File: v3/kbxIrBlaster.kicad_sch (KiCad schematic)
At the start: 46 parts, among them J1 CH1, J2 CH2, J3 CH3, J4 CH4, J5 Conn_01x06, J6 Conn_01x15, J7 Conn_01x15, J8 Barrel_Jack_Switch, J9 USB_B_Micro, Q1 2N7002, Q2 2N7002, Q3 2N7002, Q4 2N7002, SW1 RESET, SW2 BOOT, U1 TSOP382xx, U2 TSOP382xx, U3 ESP32-WROOM-32D, U4 AP2112K-3.3

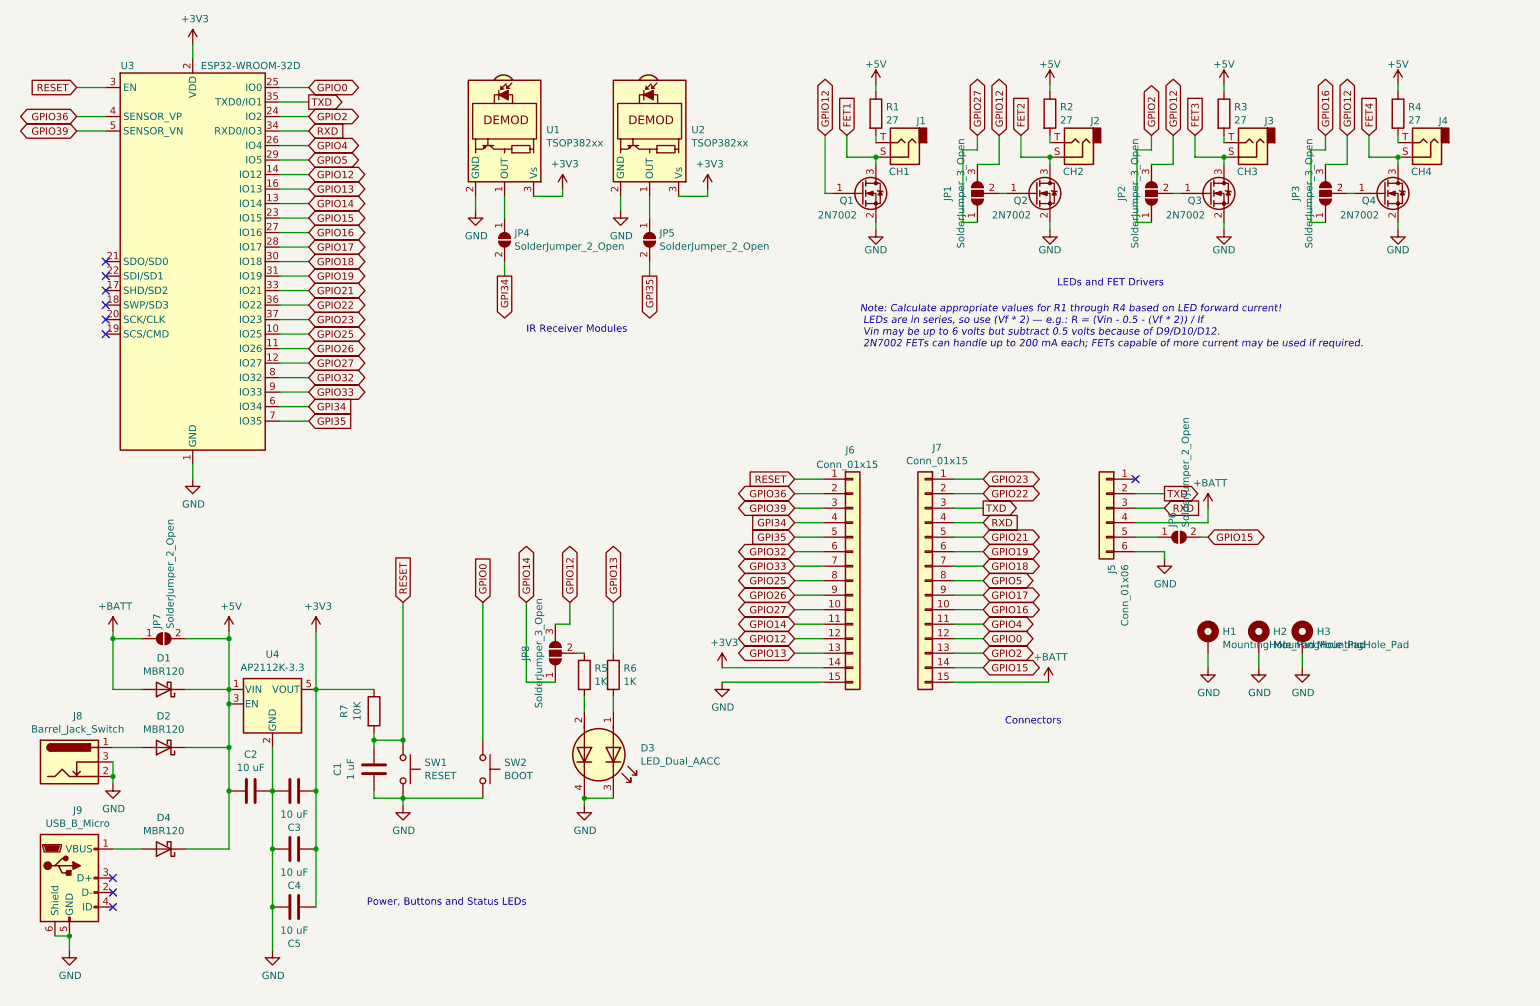
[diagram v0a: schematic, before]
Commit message: Update with v3
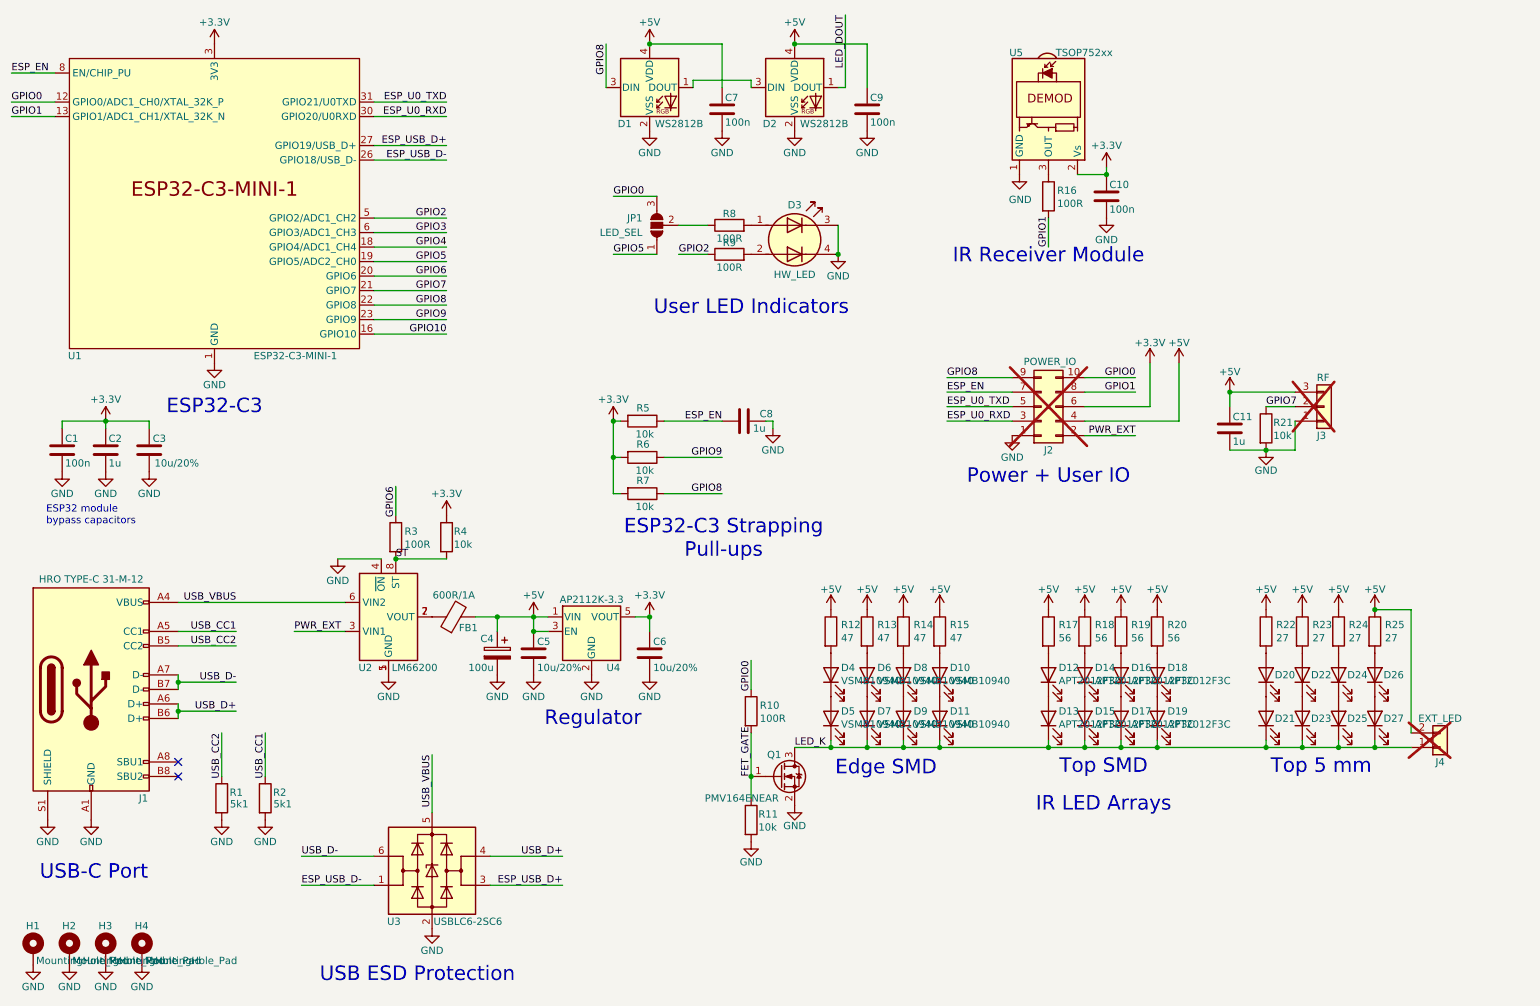
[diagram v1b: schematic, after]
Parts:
- removed C4: 10 uF, Capacitor_SMD:C_0805_2012Metric_Pad1.18x1.45mm_HandSolder, symbol Device:C
- removed D1, D2, D4: MBR120, Diode_SMD:D_SOD-123F, symbol Device:D_Schottky
- removed D3: LED_Dual_AACC, LED_SMD:LED_Cree-PLCC4_3.2x2.8mm_CCW, symbol Device:LED_Dual_AACC
- removed J1: CH1, Connector_Audio:Jack_3.5mm_CUI_SJ1-3533NG_Horizontal, symbol Connector:AudioJack2
- removed J2: CH2, Connector_Audio:Jack_3.5mm_CUI_SJ1-3533NG_Horizontal, symbol Connector:AudioJack2
- removed J3: CH3, Connector_Audio:Jack_3.5mm_CUI_SJ1-3533NG_Horizontal, symbol Connector:AudioJack2
- removed J4: CH4, Connector_Audio:Jack_3.5mm_CUI_SJ1-3533NG_Horizontal, symbol Connector:AudioJack2
- removed J5: Conn_01x06, Connector_PinHeader_2.54mm:PinHeader_1x06_P2.54mm_Vertical, symbol Connector_Generic:Conn_01x06
- removed J6, J7: Conn_01x15, Connector_PinHeader_2.54mm:PinHeader_1x15_P2.54mm_Vertical, symbol Connector_Generic:Conn_01x15
- removed J8: Barrel_Jack_Switch, Connector_BarrelJack:BarrelJack_Horizontal, symbol Connector:Barrel_Jack_Switch
- removed J9: USB_B_Micro, Connector_USB:USB_Micro-B_Molex-105017-0001, symbol Connector:USB_B_Micro
- removed JP2, JP3, JP8: SolderJumper_3_Open, Jumper:SolderJumper-3_P1.3mm_Open_RoundedPad1.0x1.5mm, symbol Jumper:SolderJumper_3_Open
- removed JP4, JP5, JP6, JP7: SolderJumper_2_Open, Jumper:SolderJumper-2_P1.3mm_Open_RoundedPad1.0x1.5mm, symbol Jumper:SolderJumper_2_Open
- removed Q2, Q3, Q4: 2N7002, Package_TO_SOT_SMD:SOT-23, symbol Transistor_FET:2N7002
- removed SW1: RESET, Button_Switch_SMD:SW_Push_1P1T_NO_CK_KMR2, symbol Switch:SW_Push
- removed SW2: BOOT, Button_Switch_SMD:SW_Push_1P1T_NO_CK_KMR2, symbol Switch:SW_Push
- removed U1, U2: TSOP382xx, OptoDevice:Vishay_MINICAST-3Pin, symbol Interface_Optical:TSOP382xx
- removed U3: ESP32-WROOM-32D, RF_Module:ESP32-WROOM-32, symbol RF_Module:ESP32-WROOM-32D
- added C10, C7, C9: 100n, Capacitor_SMD:C_0402_1005Metric, symbol Device:C
- added C11, C8: 1u, Capacitor_SMD:C_0402_1005Metric, symbol Device:C
- added C4: 100u, Capacitor_SMD:CP_Elec_5x5.4, symbol Device:CP
- added C6: 10u/20%, Capacitor_SMD:C_0603_1608Metric, symbol Device:C
- added D1, D2: WS2812B, LED_SMD:LED_WS2812B-2020_PLCC4_2.0x2.0mm, symbol Pulse:WS2812B
- added D10, D11, D4, D5, D6, D7, D8, D9: VSMB10940, LED_SMD:LED_Kingbright_KPA-3010_3x2x1mm, symbol Device:LED
- added D12, D13, D14, D15, D16, D17, D18, D19: APT2012F3C, LED_SMD:LED_0805_2012Metric, symbol Device:LED
- added D20, D21, D22, D23, D24, D25, D26, D27: CH1, LED_THT:LED_D5.0mm, symbol Device:LED
- added D3: HW_LED, LED_SMD:LED_Cree-PLCC4_3.2x2.8mm_CCW, symbol Device:LED_Dual_AAKK
- added FB1: 600R/1A, Inductor_SMD:L_0603_1608Metric, symbol Device:FerriteBead
- added H4: MountingHole_Pad, MountingHole:MountingHole_2.5mm_Pad_Via, symbol Mechanical:MountingHole_Pad
- added J1: HRO TYPE-C 31-M-12, Connector_USB:USB_C_Receptacle_HRO_TYPE-C-31-M-12, symbol Connector:USB_C_Receptacle_USB2.0
- added J2: POWER_IO, Connector_PinSocket_2.54mm:PinSocket_2x05_P2.54mm_Vertical, symbol Connector_Generic:Conn_02x05_Odd_Even
- added J3: RF, Connector_PinSocket_2.54mm:PinSocket_1x03_P2.54mm_Vertical, symbol Connector_Generic:Conn_01x03
- added J4: EXT_LED, Connector_PinSocket_2.54mm:PinSocket_1x02_P2.54mm_Vertical, symbol Connector_Generic:Conn_01x02
- added R10, R16, R8, R9: 100R, Resistor_SMD:R_0402_1005Metric, symbol Device:R
- added R11, R21: 10k, Resistor_SMD:R_0402_1005Metric, symbol Device:R
- added R12, R13, R14, R15: 47, Resistor_SMD:R_0805_2012Metric, symbol Device:R
- added R17, R18, R19, R20: 56, Resistor_SMD:R_0805_2012Metric, symbol Device:R
- added R22, R23, R24, R25: 27, Resistor_SMD:R_0805_2012Metric, symbol Device:R
- added U1: ESP32-C3-MINI-1, PCM_Espressif:ESP32-C3-MINI-1, symbol PCM_Espressif:ESP32-C3-MINI-1
- added U2: LM66200, Package_TO_SOT_SMD:SOT-583-8, symbol kbxIrBlaster:LM66200
- added U3: USBLC6-2SC6, Package_TO_SOT_SMD:SOT-23-6, symbol Power_Protection:USBLC6-2SC6
- added U5: TSOP752xx, kbxIrBlaster:Vishay_TSOP752_Horizontal, symbol kbxIrBlaster:TSOP752xx
- C1: value 1 uF -> 100n; footprint Capacitor_SMD:C_0805_2012Metric_Pad1.18x1.45mm_HandSolder -> Capacitor_SMD:C_0402_1005Metric; DesignRef (none) -> Bypass; MPN1 C0805C105K4RACTU -> CC0402KRX5R6BB104; MPN2 - -> (none); Manufacturer (none) -> Yageo
- C2: value 10 uF -> 1u; footprint Capacitor_SMD:C_0805_2012Metric_Pad1.18x1.45mm_HandSolder -> Capacitor_SMD:C_0402_1005Metric; DesignRef (none) -> Bypass; MPN1 GRM21BC81C106ME15L -> CC0402KRX5R6BB105; MPN2 - -> (none); Manufacturer (none) -> Yageo
- C3, C5: value 10 uF -> 10u/20%; footprint Capacitor_SMD:C_0805_2012Metric_Pad1.18x1.45mm_HandSolder -> Capacitor_SMD:C_0603_1608Metric; DesignRef (none) -> Bypass; MPN1 GRM21BC81C106ME15L -> CC0603MRX5R6BB106; MPN2 - -> (none); Manufacturer (none) -> Yageo
- H1, H2, H3: MPN1 - -> (none); MPN2 - -> (none)
- JP1: value SolderJumper_3_Open -> LED_SEL; footprint Jumper:SolderJumper-3_P1.3mm_Open_RoundedPad1.0x1.5mm -> Jumper:SolderJumper-3_P1.3mm_Open_RoundedPad1.0x1.5mm_NumberLabels; MPN1 - -> (none); MPN2 - -> (none); Population DNF -> (none); now left out of the parts list
- Q1: value 2N7002 -> PMV164ENEAR; MPN1 2N7002-7-F -> PMV164ENEAR; MPN2 - -> (none)
- R1, R2: value 27 -> 5k1; footprint Resistor_SMD:R_0805_2012Metric_Pad1.20x1.40mm_HandSolder -> Resistor_SMD:R_0402_1005Metric; DesignRef (none) -> USB-C CC line pull resistors; MPN1 RC0805FR-0727RL -> RC0402JR-075K1L; MPN2 - -> (none); Manufacturer (none) -> Yageo
- R3: value 27 -> 100R; footprint Resistor_SMD:R_0805_2012Metric_Pad1.20x1.40mm_HandSolder -> Resistor_SMD:R_0402_1005Metric; MPN1 RC0805FR-0727RL -> RC0402JR-07100RL; MPN2 - -> (none); Manufacturer (none) -> Yageo
- R4: value 27 -> 10k; footprint Resistor_SMD:R_0805_2012Metric_Pad1.20x1.40mm_HandSolder -> Resistor_SMD:R_0402_1005Metric; DesignRef (none) -> Pull-up; MPN1 RC0805FR-0727RL -> RC0402JR-0710KL; MPN2 - -> (none); Manufacturer (none) -> Yageo
- R5, R6: value 1K -> 10k; footprint Resistor_SMD:R_0805_2012Metric_Pad1.20x1.40mm_HandSolder -> Resistor_SMD:R_0402_1005Metric; DesignRef (none) -> Pull-up; MPN1 RC0805FR-071KL -> RC0402JR-0710KL; MPN2 - -> (none); Manufacturer (none) -> Yageo
- R7: value 10K -> 10k; footprint Resistor_SMD:R_0805_2012Metric_Pad1.20x1.40mm_HandSolder -> Resistor_SMD:R_0402_1005Metric; DesignRef (none) -> Pull-up; MPN1 RC0805FR-0710KL -> RC0402JR-0710KL; MPN2 - -> (none); Manufacturer (none) -> Yageo
- U4: MPN2 - -> (none)
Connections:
- net GPIO27 is gone; now on net GPIO5: JP1.1 (A)
- net RESET is gone; now on net +3.3V: C1.1, R7.2
- net +5V: now also C5.1, C11.1, C4.1, C7.1, C9.1, D1.4 (VDD), D2.4 (VDD), FB1.2, J2.4 (Pin_4), J3.3 (Pin_3), J4.2 (Pin_2), R12.1, R13.1, R14.1, R15.1, R17.1, R18.1, R19.1, R20.1, R22.1, R23.1, R24.1, R25.1; no longer C2.2, R1.1, R2.1, R3.1, R4.1
- net GND: now also C2.2, C3.2, C5.2, R1.2, R2.2, C10.2, C11.2, C4.2, C6.2, C7.2, C8.2, C9.2, D1.2 (VSS), D2.2 (VSS), D3.3 (K1), D3.4 (K2), H4.1, J1.A1 (GND), J1.A12 (GND), J1.B1 (GND), J1.B12 (GND), J1.S1 (SHIELD), J2.1 (Pin_1), J3.1 (Pin_1), R11.2, R21.2, U1.1 (GND), U1.11 (GND), U1.14 (GND), U1.2 (GND), U1.36 (GND), U1.37 (GND), U1.38 (GND), U1.39 (GND), U1.40 (GND), U1.41 (GND), U1.42 (GND), U1.43 (GND), U1.44 (GND), U1.45 (GND), U1.46 (GND), U1.47 (GND), U1.48 (GND), U1.49 (GND), U1.50 (GND), U1.51 (GND), U1.52 (GND), U1.53 (GND), U2.1 (GND), U2.4 (~{ON}), U2.5 (GND), U3.2 (GND), U5.1 (GND), U5.4 (GND); no longer C2.1, C3.1, C5.1
- net GPIO0: now also JP1.3 (B), J2.10 (Pin_10), R10.1, U1.12 (GPIO0/ADC1_CH0/XTAL_32K_P)
- net GPIO2: now also R9.1, U1.5 (GPIO2/ADC1_CH2)
- net GPIO4: now also U1.18 (GPIO4/ADC1_CH4)
- net GPIO5: now also U1.19 (GPIO5/ADC2_CH0)
- net +3.3V: now reaches R6.2
- net +3.3V: now also C2.1, C3.1, R4.1, R5.2, U4.5 (VOUT), C10.1, C6.1, J2.6 (Pin_6), U1.3 (3V3), U5.2 (Vs)
- net ESP_EN: now reaches R5.1
- net ESP_EN: now also C8.1, J2.7 (Pin_7), U1.8 (EN/CHIP_PU)
- net at JP1.2 (C): now also R8.1
- net ST: now reaches R3.2
- net ST: now also R4.2, U2.8 (ST)
- removed net +3V3: C3.2, C5.2, R7.1, U4.5 (VOUT)
- net FET1 renamed LED_K
- net LED_K: now also D11.1 (K), D13.1 (K), D15.1 (K), D17.1 (K), D19.1 (K), D21.1 (K), D23.1 (K), D25.1 (K), D27.1 (K), D5.1 (K), D7.1 (K), D9.1 (K), J4.1 (Pin_1)
- net GPIO12 renamed FET_GATE
- net FET_GATE: now also R10.2, R11.1; no longer JP1.3 (B)
- net GPIO13 renamed GPIO9
- net GPIO9: now also U1.23 (GPIO9)
- new net: D1.1 (DOUT), D2.3 (DIN)
- new net: D18.2 (A), R20.2
- new net: D3.2 (A2), R9.2
- new net: D22.1 (K), D23.2 (A)
- new net: D22.2 (A), R23.2
- new net: R16.1, U5.3 (OUT)
- new net: D20.2 (A), R22.2
- new net: D16.1 (K), D17.2 (A)
- new net: D16.2 (A), R19.2
- new net: D6.1 (K), D7.2 (A)
- new net: D6.2 (A), R13.2
- new net: D12.1 (K), D13.2 (A)
- new net: D14.2 (A), R18.2
- new net: D24.1 (K), D25.2 (A)
- new net: D3.1 (A1), R8.2
- new net: D4.1 (K), D5.2 (A)
- new net: FB1.1, U2.2 (VOUT), U2.7 (VOUT)
- new net: D10.2 (A), R15.2
- new net: D18.1 (K), D19.2 (A)
- new net: D26.2 (A), R25.2
- new net: D24.2 (A), R24.2
- new net: D20.1 (K), D21.2 (A)
- new net: D8.1 (K), D9.2 (A)
- new net: D8.2 (A), R14.2
- new net: D26.1 (K), D27.2 (A)
- new net: D10.1 (K), D11.2 (A)
- new net: D4.2 (A), R12.2
- new net: D12.2 (A), R17.2
- new net: D14.1 (K), D15.2 (A)
- new net ESP_U0_RXD: J2.3 (Pin_3), U1.30 (GPIO20/U0RXD)
- new net ESP_U0_TXD: J2.5 (Pin_5), U1.31 (GPIO21/U0TXD)
- new net ESP_USB_D+: U1.27 (GPIO19/USB_D+), U3.3 (I/O2)
- new net ESP_USB_D-: U1.26 (GPIO18/USB_D-), U3.1 (I/O1)
- new net GPIO1: J2.8 (Pin_8), R16.2, U1.13 (GPIO1/ADC1_CH1/XTAL_32K_N)
- new net GPIO10: U1.16 (GPIO10)
- new net GPIO3: U1.6 (GPIO3/ADC1_CH3)
- new net GPIO6: R3.1, U1.20 (GPIO6)
- new net GPIO7: J3.2 (Pin_2), R21.1, U1.21 (GPIO7)
- new net GPIO8: D1.3 (DIN), J2.9 (Pin_9), R7.1, U1.22 (GPIO8)
- new net LED_DOUT: D2.1 (DOUT)
- new net PWR_EXT: J2.2 (Pin_2), U2.3 (VIN1)
- new net USB_CC1: J1.A5 (CC1), R2.1
- new net USB_CC2: J1.B5 (CC2), R1.1
- new net USB_D+: J1.A6 (D+), J1.B6 (D+), U3.4 (I/O2)
- new net USB_D-: J1.A7 (D-), J1.B7 (D-), U3.6 (I/O1)
- new net USB_VBUS: J1.A4 (VBUS), J1.A9 (VBUS), J1.B4 (VBUS), J1.B9 (VBUS), U2.6 (VIN2), U3.5 (VBUS)
- no-connect marks 10 -> 2
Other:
- note added: "ESP32 module bypass capacitors"
- note added: "ESP32-C3"
- note added: "ESP32-C3 Strapping Pull-ups"
- note added: "Edge SMD"
- note added: "IR LED Arrays"
- note added: "IR Receiver Module"
- note added: "Power + User IO"
- note added: "Regulator"
- note added: "Top 5 mm"
- note added: "Top SMD"
- note added: "USB ESD Protection"
- note added: "USB-C Port"
- note added: "User LED Indicators"
- note removed: "Connectors"
- note removed: "IR Receiver Modules"
- note removed: "LEDs and FET Drivers"
- note removed: "Note: Calculate appropriate values for R1 through R4 based on LED forward current! LEDs are in series, so use (Vf * 2) — e.g.: R = (Vin - 0.5 - (Vf * 2)) / If Vin may be up to 6 volts but subtract 0.5 volts because of D9/D10/D12. 2N7002 FETs can handle up to 200 mA each; FETs capable of more current may be used if required."
- note removed: "Power, Buttons and Status LEDs"
- moved on the sheet: H1, Q1, U4
